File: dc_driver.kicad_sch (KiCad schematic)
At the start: 36 parts, among them U2 L298N, U3 L298N, U4 L298N

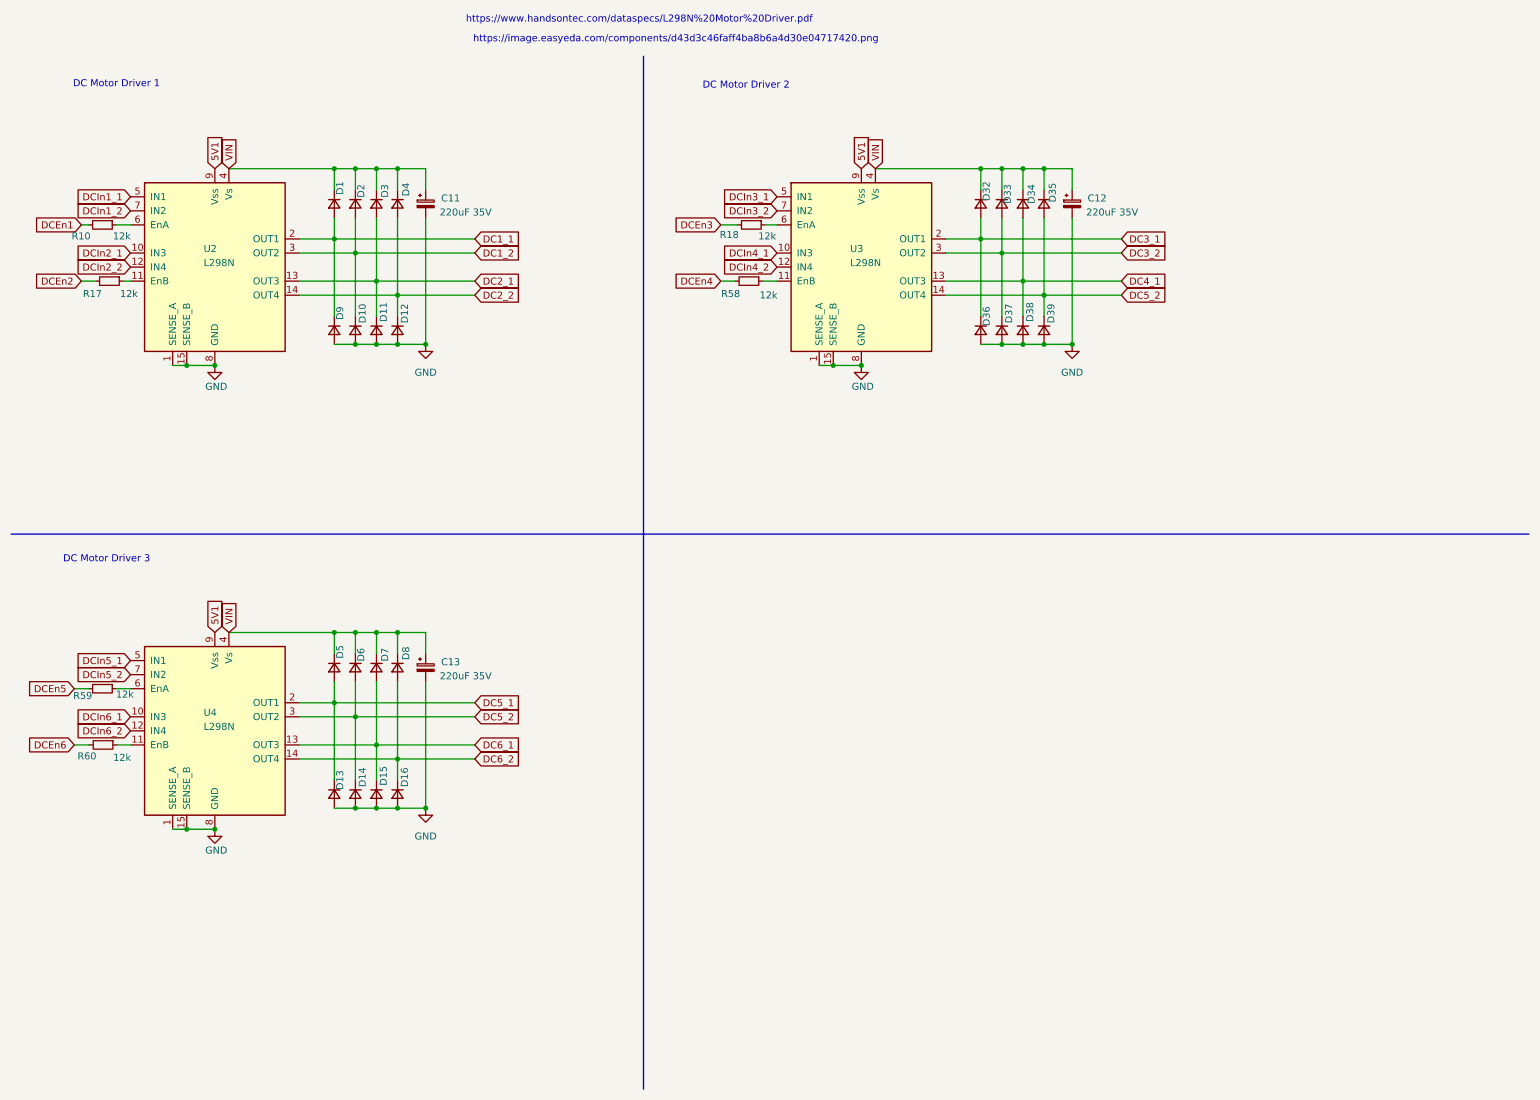
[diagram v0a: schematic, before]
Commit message: esp32 silindi, yerleştirmeler yapıldı
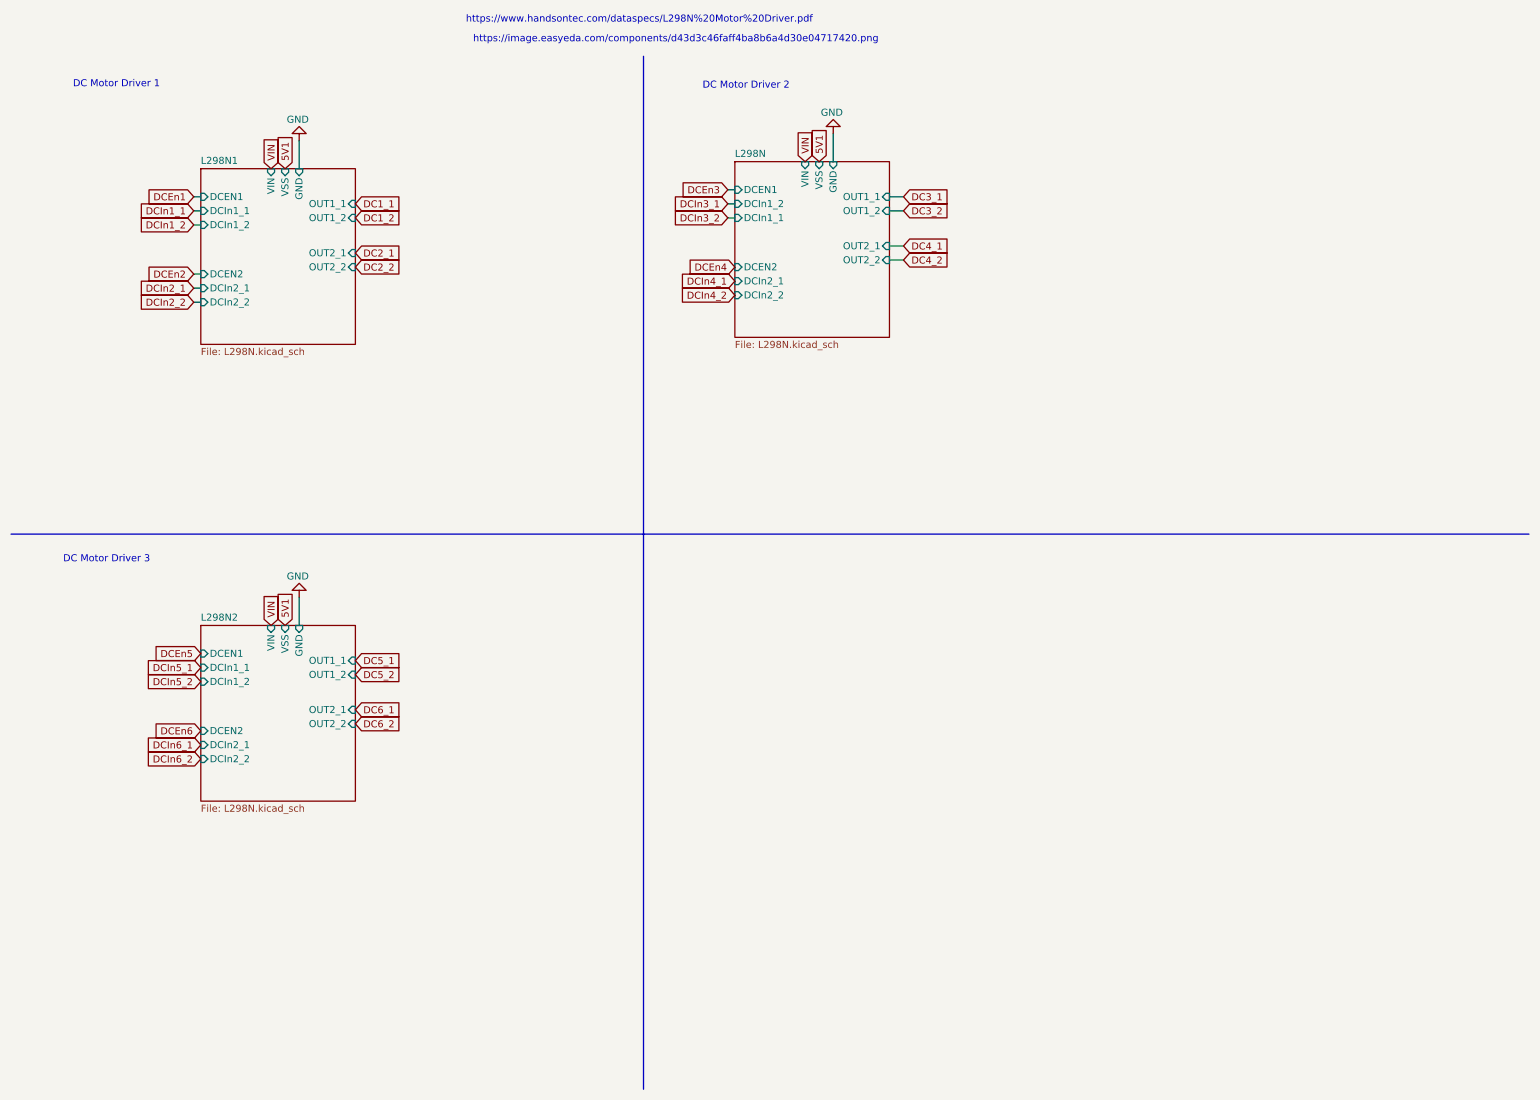
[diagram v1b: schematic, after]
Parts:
- removed C11, C12, C13: 220uF 35V, Capacitor_SMD:CP_Elec_8x10.5, symbol Device:C_Polarized_Small
- removed D1, D10, D11, D12, D13, D14, D15, D16, D2, D3, D32, D33, D34, D35, D36, D37, D38, D39, D4, D5, D6, D7, D8, D9: 1N4007, Diode_SMD:D_SOD-123, symbol Device:D_Small
- removed R10, R17, R18, R58, R59, R60: 12k, Resistor_SMD:R_0805_2012Metric, symbol Device:R_Small
- removed U2, U3, U4: L298N, Package_TO_SOT_THT:TO-220-15_P2.54x2.54mm_StaggerOdd_Lead4.58mm_Vertical, symbol Driver_Motor:L298N
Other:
- added sheet L298N (L298N.kicad_sch)
- added sheet L298N1 (L298N.kicad_sch)
- added sheet L298N2 (L298N.kicad_sch)
